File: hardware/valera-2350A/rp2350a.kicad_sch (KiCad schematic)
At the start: 25 parts, among them SW1 Flash Button, Y1 12 MHz

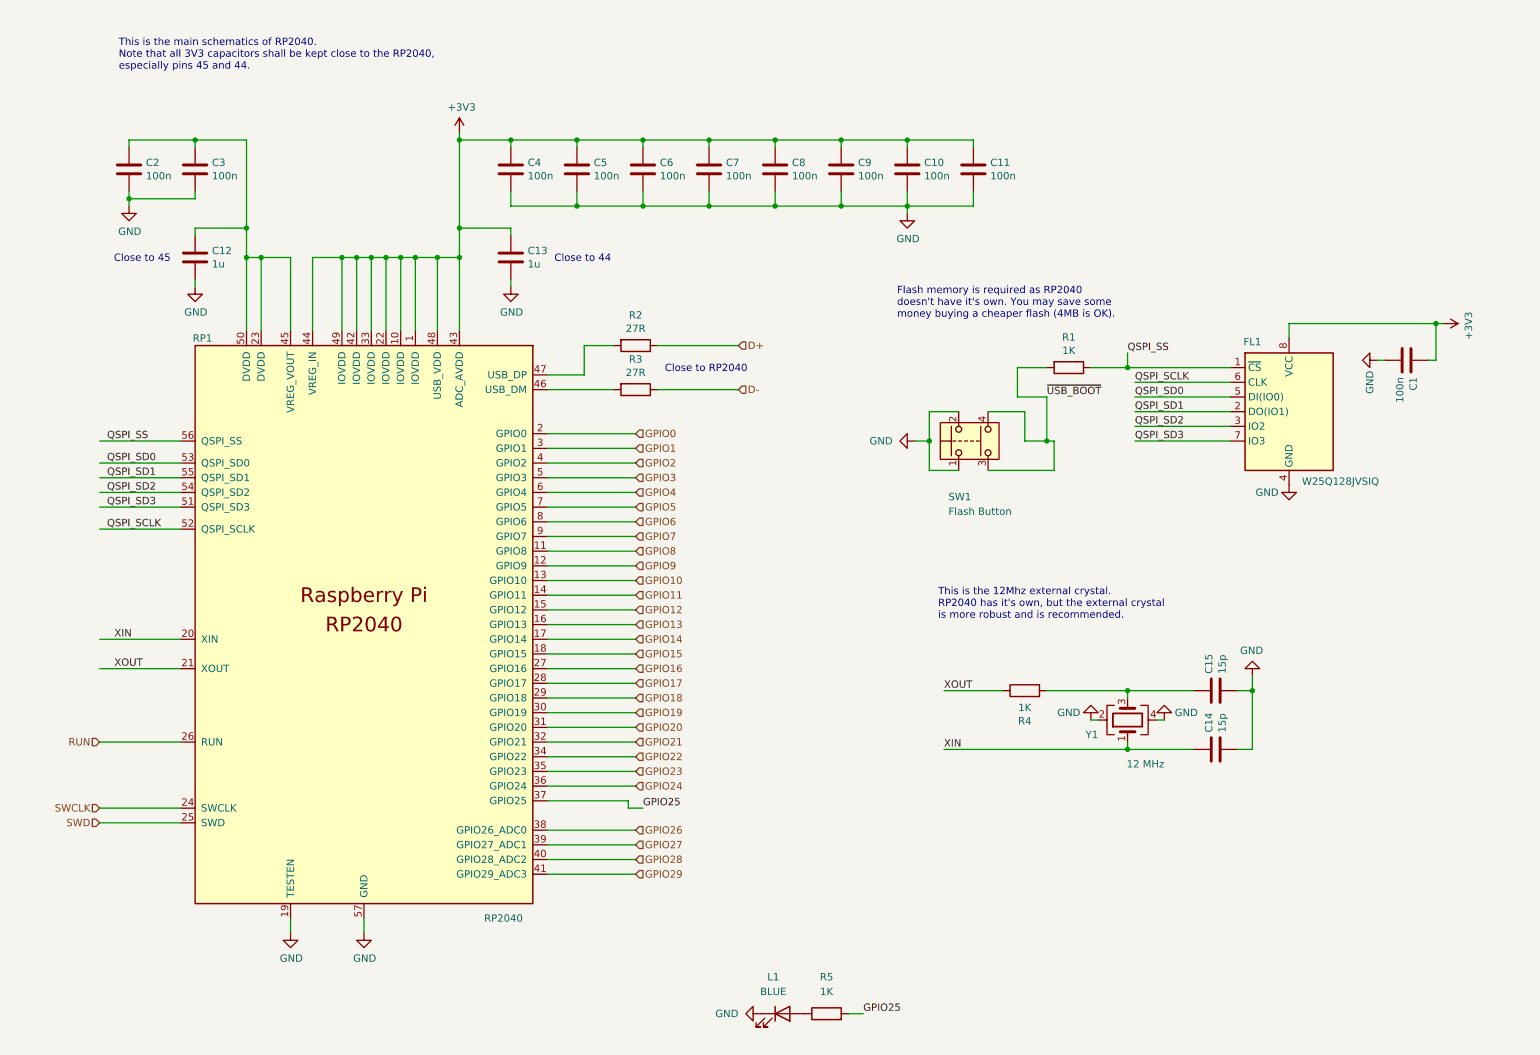
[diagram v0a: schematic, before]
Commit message: HW Rev 1.0 work-in-progress
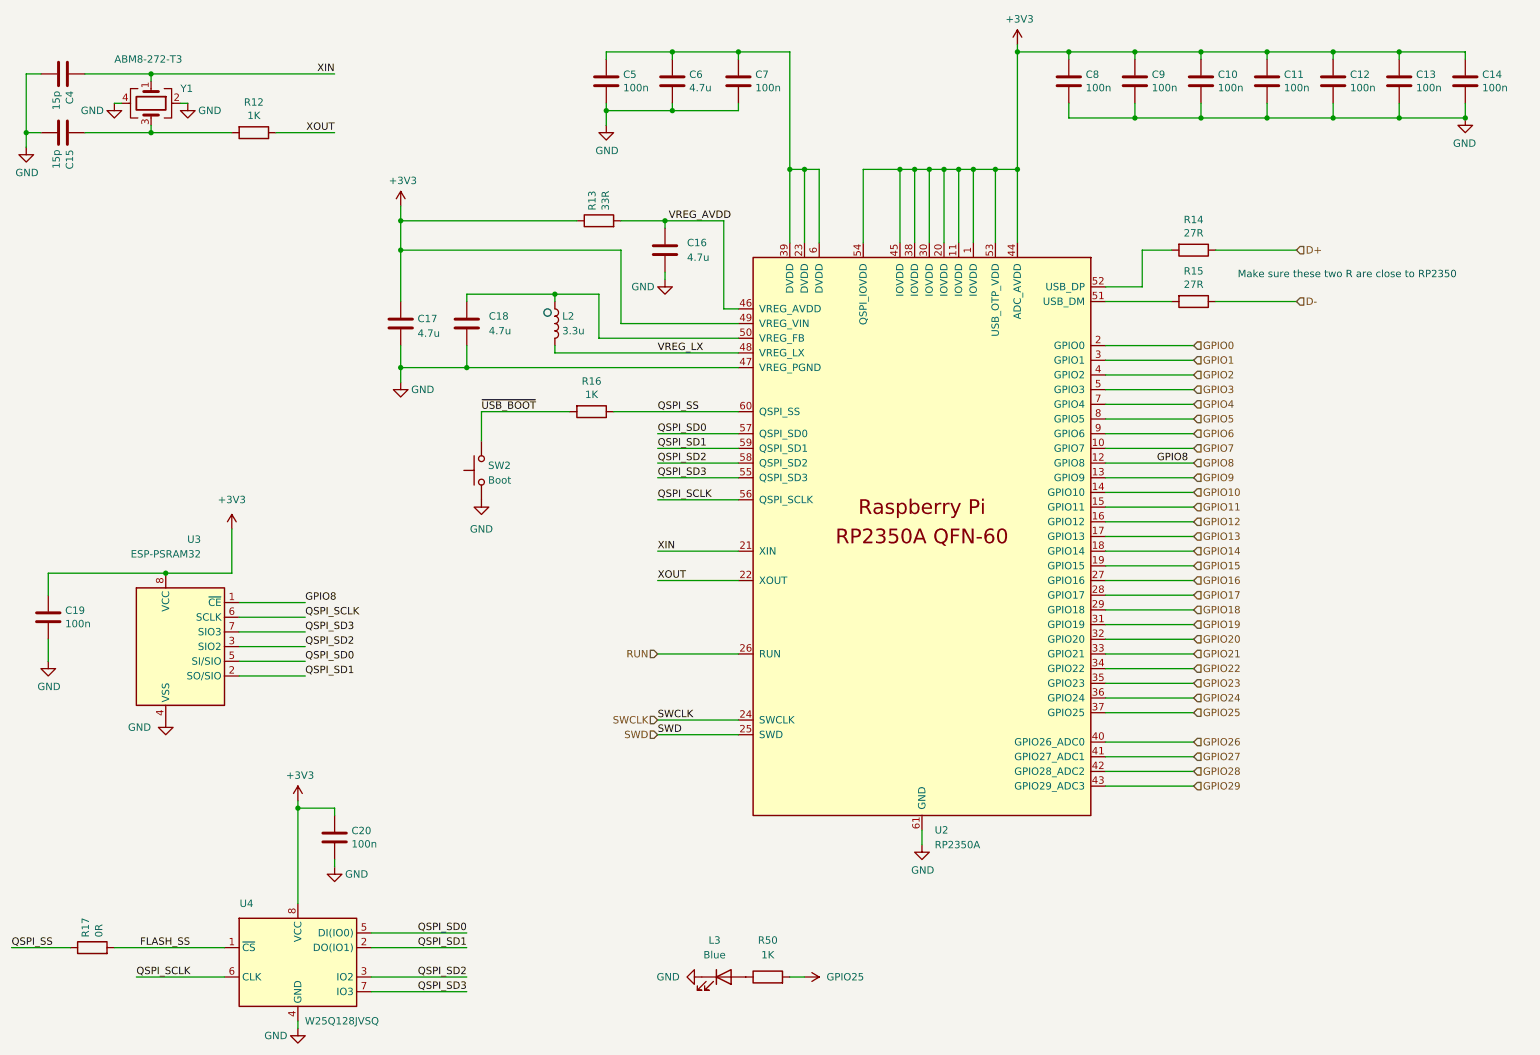
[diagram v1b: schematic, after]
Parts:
- removed C1, C2, C3: 100n, FRANK:Capacitor (0805), symbol Device:C
- removed FL1: W25Q128JVSIQ, FRANK:SOIC-8, symbol FRANK:Flash_W25Q128JVS
- removed L1: BLUE, FRANK:LED (0805), symbol Device:LED
- removed R1, R4, R5: 1K, FRANK:Resistor (0805), symbol Device:R
- removed R2, R3: 27R, FRANK:Resistor (0805), symbol Device:R
- removed RP1: RP2040, FRANK:QFN 56, symbol FRANK:RP2040
- removed SW1: Flash Button, FRANK:Button (SMD, 3x3mm), symbol Switch:SW_Push_Dual
- added C16, C17, C18: 4.7u, FRANK:Capacitor (0805), symbol Device:C
- added C19, C20: 100n, FRANK:Capacitor (0805), symbol Device:C
- added L2: 3.3u, FRANK:Inductor (3225), symbol Device:L
- added L3: Blue, FRANK:LED (0805), symbol Device:LED
- added R12, R16, R50: 1K, FRANK:Resistor (0805), symbol Device:R
- added R13: 33R, FRANK:Resistor (0805), symbol Device:R
- added R14, R15: 27R, FRANK:Resistor (0805), symbol Device:R
- added R17: 0R, FRANK:Resistor (0805), symbol Device:R
- added SW2: Boot, FRANK:Button (SMD, 3x3mm, 1-1), symbol Switch:SW_Push
- added U2: RP2350A, FRANK:QFN 60 (RP2350A), symbol FRANK:RP2350A
- added U3: ESP-PSRAM32, FRANK:SOIC-8, symbol FRANK:ESP-PSRAM32
- added U4: W25Q128JVSQ, FRANK:SOIC-8, symbol FRANK:W25Q128JVS
- C10, C11, C15, C5, C7, C8, C9: AliExpress https://www.aliexpress.com/item/33008008276.html -> (none)
- C12, C13: value 1u -> 100n; AliExpress https://www.aliexpress.com/item/33008008276.html -> (none)
- C14: value 15p -> 100n; AliExpress https://www.aliexpress.com/item/33008008276.html -> (none)
- C4: value 100n -> 15p; AliExpress https://www.aliexpress.com/item/33008008276.html -> (none)
- C6: value 100n -> 4.7u; AliExpress https://www.aliexpress.com/item/33008008276.html -> (none)
- Y1: value 12 MHz -> ABM8-272-T3; AliExpress https://www.aliexpress.com/item/1005004661413307.html -> (none)
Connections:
- net +3V3: now also C12.1, C14.1, C17.1, C19.1, C20.1, R13.1, U2.1 (IOVDD), U2.11 (IOVDD), U2.20 (IOVDD), U2.30 (IOVDD), U2.38 (IOVDD), U2.44 (ADC_AVDD), U2.45 (IOVDD), U2.49 (VREG_VIN), U2.53 (USB_OTP_VDD), U2.54 (QSPI_IOVDD), U3.8 (VCC), U4.8 (VCC); no longer C4.1, C5.1, C6.1, C7.1
- net D+: now also R14.1
- net D-: now also R15.1
- net GND: now also C16.2, C17.2, C18.2, C19.2, C20.2, L3.1 (K), SW2.1, U2.47 (VREG_PGND), U2.61 (GND), U3.4 (VSS), U4.4 (GND)
- net GPIO0: now also U2.2 (GPIO0)
- net GPIO1: now also U2.3 (GPIO1)
- net GPIO10: now also U2.14 (GPIO10)
- net GPIO11: now also U2.15 (GPIO11)
- net GPIO12: now also U2.16 (GPIO12)
- net GPIO13: now also U2.17 (GPIO13)
- net GPIO14: now also U2.18 (GPIO14)
- net GPIO15: now also U2.19 (GPIO15)
- net GPIO16: now also U2.27 (GPIO16)
- net GPIO17: now also U2.28 (GPIO17)
- net GPIO18: now also U2.29 (GPIO18)
- net GPIO19: now also U2.31 (GPIO19)
- net GPIO2: now also U2.4 (GPIO2)
- net GPIO20: now also U2.32 (GPIO20)
- net GPIO21: now also U2.33 (GPIO21)
- net GPIO22: now also U2.34 (GPIO22)
- net GPIO23: now also U2.35 (GPIO23)
- net GPIO24: now also U2.36 (GPIO24)
- net GPIO25: now also R50.2, U2.37 (GPIO25)
- net GPIO26: now also U2.40 (GPIO26_ADC0)
- net GPIO27: now also U2.41 (GPIO27_ADC1)
- net GPIO28: now also U2.42 (GPIO28_ADC2)
- net GPIO29: now also U2.43 (GPIO29_ADC3)
- net GPIO3: now also U2.5 (GPIO3)
- net GPIO4: now also U2.7 (GPIO4)
- net GPIO5: now also U2.8 (GPIO5)
- net GPIO6: now also U2.9 (GPIO6)
- net GPIO7: now also U2.10 (GPIO7)
- net GPIO8: now also U2.12 (GPIO8), U3.1 (~{CE})
- net GPIO9: now also U2.13 (GPIO9)
- net QSPI_SCLK: now also U2.56 (QSPI_SCLK), U3.6 (SCLK), U4.6 (CLK)
- net QSPI_SD0: now also U2.57 (QSPI_SD0), U3.5 (SI/SIO), U4.5 (DI(IO0))
- net QSPI_SD1: now also U2.59 (QSPI_SD1), U3.2 (SO/SIO), U4.2 (DO(IO1))
- net QSPI_SD2: now also U2.58 (QSPI_SD2), U3.3 (SIO2), U4.3 (IO2)
- net QSPI_SD3: now also U2.55 (QSPI_SD3), U3.7 (SIO3), U4.7 (IO3)
- net QSPI_SS: now also R16.1, R17.1, U2.60 (QSPI_SS)
- net RUN: now also U2.26 (RUN)
- net SWCLK: now also U2.24 (SWCLK)
- net SWD: now also U2.25 (SWD)
- net XIN: now also C4.1, U2.21 (XIN); no longer C14.1
- net XOUT: now also R12.1, U2.22 (XOUT)
- net ~{USB_BOOT}: now also R16.2, SW2.2
- net at C15.1, Y1.3: now also R12.2
- new net: C18.1, L2.1, U2.50 (VREG_FB)
- new net: C5.1, C6.1, C7.1, U2.23 (DVDD), U2.39 (DVDD), U2.6 (DVDD)
- new net: R14.2, U2.52 (USB_DP)
- new net: L3.2 (A), R50.1
- new net: R15.2, U2.51 (USB_DM)
- new net FLASH_SS: R17.2, U4.1 (~{CS})
- new net VREG_AVDD: C16.1, R13.2, U2.46 (VREG_AVDD)
- new net VREG_LX: L2.2, U2.48 (VREG_LX)
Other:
- note added: "Make sure these two R are close to RP2350"
- note removed: "Close to 44"
- note removed: "Close to 45"
- note removed: "Close to RP2040"
- note removed: "Flash memory is required as RP2040 doesn't have it's own. You may save some money buying a cheaper flash (4MB is OK)."
- note removed: "This is the 12Mhz external crystal. RP2040 has it's own, but the external crystal is more robust and is recommended."
- note removed: "This is the main schematics of RP2040. Note that all 3V3 capacitors shall be kept close to the RP2040, especially pins 45 and 44."
